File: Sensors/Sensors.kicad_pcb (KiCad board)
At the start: 2 copper layers, 92.5 x 55 mm, 19 parts, among them IC1 CD4051B, J2 Conn_01x06, Q1 TCRT5000, Q2 TCRT5000, Q3 TCRT5000, Q4 TCRT5000, Q5 TCRT5000, Q6 TCRT5000, Q7 TCRT5000, Q8 TCRT5000

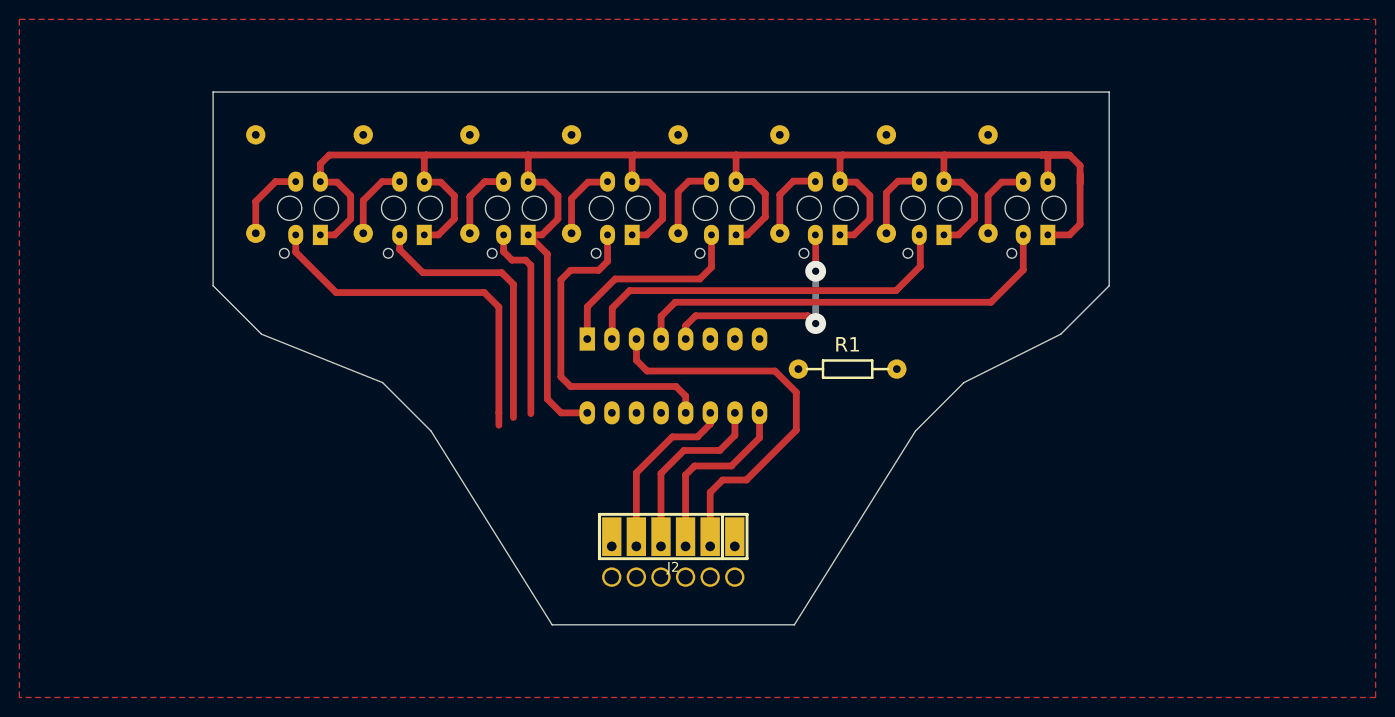
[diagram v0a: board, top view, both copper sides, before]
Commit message: Rev. 1.0.0
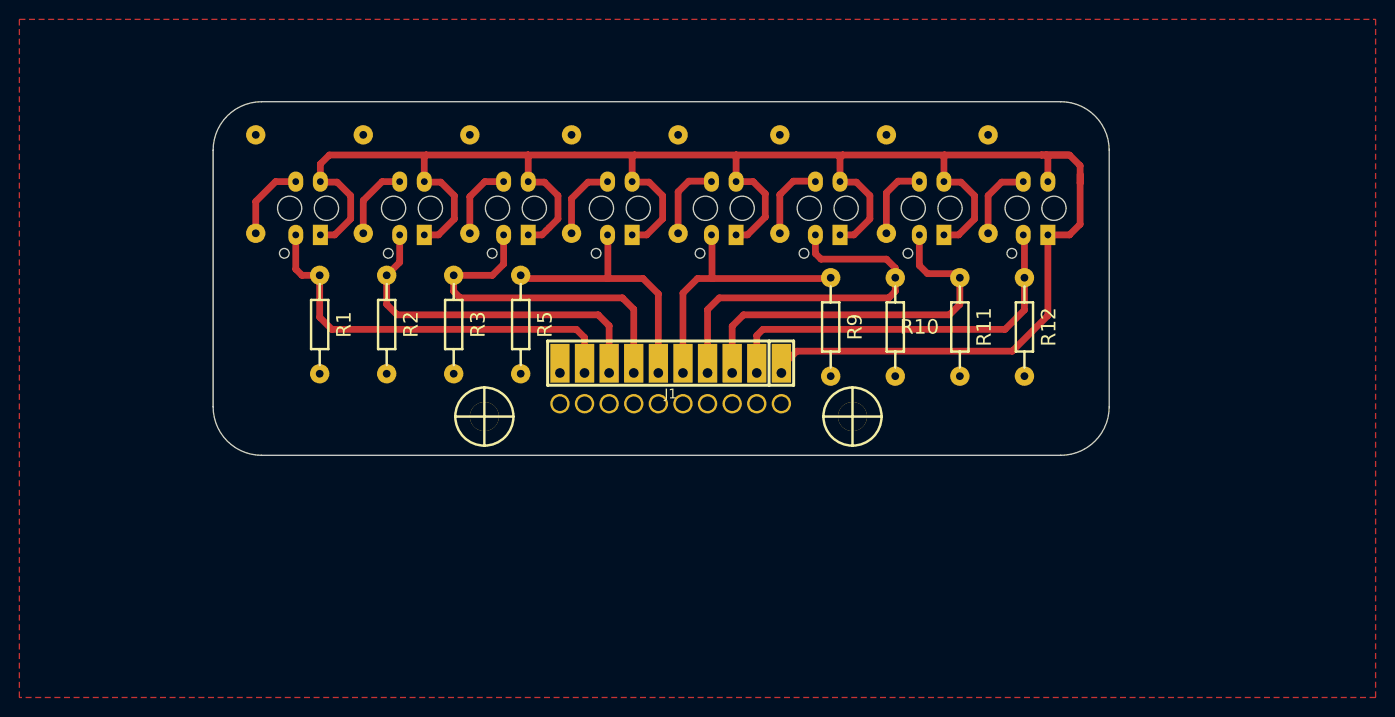
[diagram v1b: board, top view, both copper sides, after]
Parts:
- removed IC1: CD4051B, MacroLib:DIP-16
- added J1: CONN_01X10, MacroLib:Pin_Header_Wire_10, F.Cu at (142.2, 111.5)
- added J3: Cable_PAD, EESTN5:Tornillo_M3_8mm, F.Cu at (123.0, 116.0)
- added R10: R, MacroLib:RES0.3, F.Cu at (165.4, 106.8)
- added R11: R, MacroLib:RES0.3, F.Cu at (172.1, 106.8)
- added R12: R, MacroLib:RES0.3, F.Cu at (178.8, 106.8)
- added R2: R, MacroLib:RES0.3, F.Cu at (112.9, 106.5)
- added R3: R, MacroLib:RES0.3, F.Cu at (119.8, 106.5)
- added R5: R, MacroLib:RES0.3, F.Cu at (126.8, 106.5)
- added R9: R, MacroLib:RES0.3, F.Cu at (158.8, 106.8)
- J2: value Conn_01x06 -> Cable_PAD; footprint MacroLib:Pin_Header_Wire_6 -> EESTN5:Tornillo_M3_8mm
- R1: value 10k -> R
- moved R1 54.7 mm to (106.0, 106.5), turned to -90 degrees
- moved J2 22.8 mm to (161.0, 116.0), turned to 0 degrees
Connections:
- J2 pad 1: GND -> unconnected-(J2-Pad1)
- R1 pad 1: /COM -> /CH_0
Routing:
- net /COM: track 41.4 -> 0.00 mm
- net /C: track 19.2 -> 0.00 mm
- net /B: track 19.1 -> 0.00 mm
- net /A: track 18.5 -> 0.00 mm
- net VCC: track 205.7 -> 221.9 mm
- net /CH_2: track 20.4 -> 36.2 mm
- net /CH_5: track 24.7 -> 39.9 mm, vias 2 -> 0
- net /CH_1: track 28.5 -> 36.5 mm
- net /CH_4: track 21.2 -> 28.7 mm
- net /CH_3: track 33.8 -> 27.7 mm
- net /CH_0: track 37.3 -> 42.5 mm
- net /CH_7: track 45.3 -> 40.4 mm
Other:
- board size 92.5 x 55 mm -> 92.5 x 36.5 mm
- board text removed: "${REFERENCE}"
